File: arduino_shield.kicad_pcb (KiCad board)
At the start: 2 copper layers, 59.1 x 53.3 mm, 33 parts, among them P1 Power, P2 Analog, P3 Digital, P4 Digital, P5 CONN_01X01, P6 CONN_01X01, P7 CONN_01X01, P8 CONN_01X01, U1 MS560702BA03-50

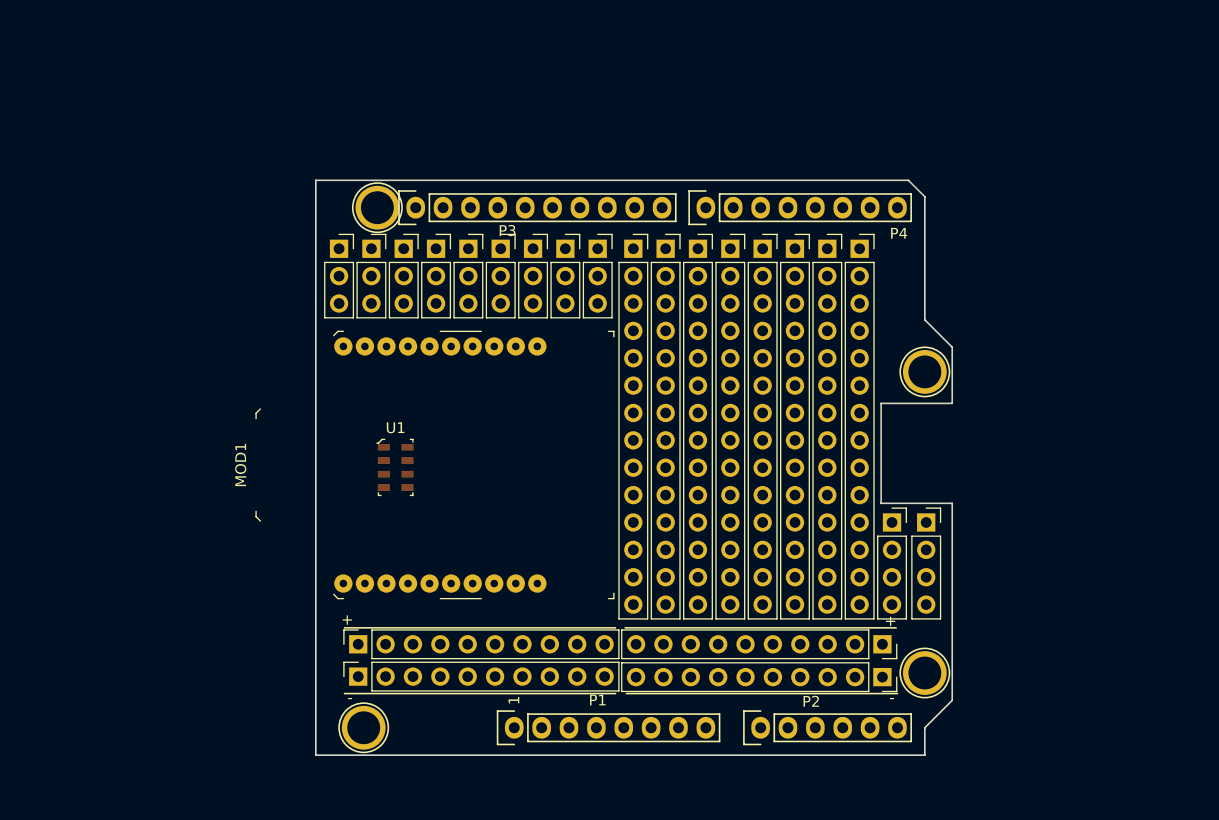
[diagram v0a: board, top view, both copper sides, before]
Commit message: finished maybe?
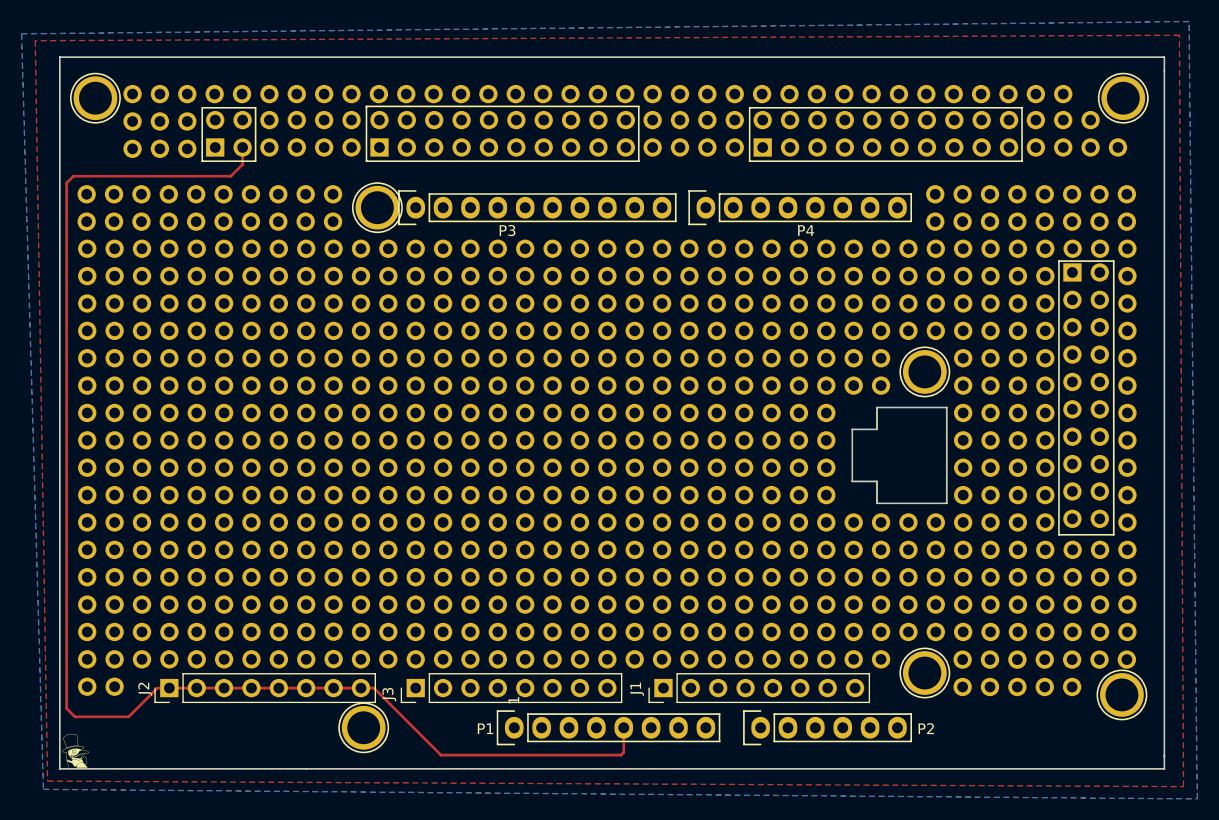
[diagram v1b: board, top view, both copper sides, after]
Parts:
- removed MOD1: XBP9B-DMST-002, digikey-footprints:XBEE_PRO-20_THT
- removed the REF** at (177.2, 104.8)
- removed the REF** at (137.7, 79.4)
- removed the REF** at (134.7, 79.4)
- removed the REF** at (131.7, 79.4)
- removed the REF** at (128.7, 79.4)
- removed the REF** at (125.7, 79.4)
- removed the REF** at (171.0, 79.4)
- removed the REF** at (168.0, 79.4)
- removed the REF** at (165.0, 79.4)
- removed the REF** at (162.0, 79.4)
- removed the REF** at (159.0, 79.4)
- removed the REF** at (174.0, 104.8)
- removed the REF** at (156.0, 79.4)
- removed the REF** at (153.0, 79.4)
- removed the REF** at (150.0, 79.4)
- removed the REF** at (122.7, 79.4)
- removed the REF** at (173.1, 116.1)
- removed the REF** at (173.1, 119.1)
- removed the REF** at (124.5, 119.1)
- removed the REF** at (124.5, 116.1)
- removed the REF** at (146.7, 79.4)
- removed the REF** at (143.7, 79.4)
- removed the REF** at (140.7, 79.4)
- added G***: LOGO, penguin:test106, F.Cu at (98.7, 126.0)
- added J1: GND Rail, Connector_PinHeader_2.54mm:PinHeader_1x08_P2.54mm_Vertical, F.Cu at (152.8, 120.1)
- added J2: 5V Rail, Connector_PinHeader_2.54mm:PinHeader_1x08_P2.54mm_Vertical, F.Cu at (106.9, 120.1)
- added J3: 3v3 Rail, Connector_PinHeader_2.54mm:PinHeader_1x08_P2.54mm_Vertical, F.Cu at (129.8, 120.1)
- added P7: CONN_01X01, Socket_Arduino_Uno:Arduino_1pin, F.Cu at (195.3, 120.8)
- added P7: CONN_01X01, Socket_Arduino_Uno:Arduino_1pin, F.Cu at (195.5, 65.4)
- added P7: CONN_01X01, Socket_Arduino_Uno:Arduino_1pin, F.Cu at (100.1, 65.4)
- added REF**: PROTO_HOLE, One_Month_Footprints:PROTO_HOLE, F.Cu at (101.9, 120.0)
- added REF**: PROTO_HOLE, One_Month_Footprints:PROTO_HOLE, F.Cu at (114.5, 76.9)
- added REF**: PROTO_HOLE, One_Month_Footprints:PROTO_HOLE, F.Cu at (112.0, 97.2)
- added REF**: PROTO_HOLE, One_Month_Footprints:PROTO_HOLE, F.Cu at (109.5, 97.2)
- added REF**: PROTO_HOLE, One_Month_Footprints:PROTO_HOLE, F.Cu at (106.9, 97.2)
- added REF**: PROTO_HOLE, One_Month_Footprints:PROTO_HOLE, F.Cu at (104.4, 97.2)
- added REF**: PROTO_HOLE, One_Month_Footprints:PROTO_HOLE, F.Cu at (101.9, 97.2)
- added REF**: PROTO_HOLE, One_Month_Footprints:PROTO_HOLE, F.Cu at (99.3, 97.2)
- added REF**: PROTO_HOLE, One_Month_Footprints:PROTO_HOLE, F.Cu at (119.6, 94.6)
- added REF**: PROTO_HOLE, One_Month_Footprints:PROTO_HOLE, F.Cu at (117.1, 94.6)
- added REF**: PROTO_HOLE, One_Month_Footprints:PROTO_HOLE, F.Cu at (114.6, 94.6)
- added REF**: PROTO_HOLE, One_Month_Footprints:PROTO_HOLE, F.Cu at (112.0, 94.6)
- added REF**: PROTO_HOLE, One_Month_Footprints:PROTO_HOLE, F.Cu at (109.4, 76.9)
- added REF**: PROTO_HOLE, One_Month_Footprints:PROTO_HOLE, F.Cu at (109.5, 94.6)
- added REF**: PROTO_HOLE, One_Month_Footprints:PROTO_HOLE, F.Cu at (106.9, 94.6)
- added REF**: PROTO_HOLE, One_Month_Footprints:PROTO_HOLE, F.Cu at (104.4, 94.6)
- added REF**: PROTO_HOLE, One_Month_Footprints:PROTO_HOLE, F.Cu at (101.9, 94.6)
- added REF**: PROTO_HOLE, One_Month_Footprints:PROTO_HOLE, F.Cu at (99.3, 94.6)
- added REF**: PROTO_HOLE, One_Month_Footprints:PROTO_HOLE, F.Cu at (119.6, 92.1)
- added REF**: PROTO_HOLE, One_Month_Footprints:PROTO_HOLE, F.Cu at (117.1, 92.1)
- added REF**: PROTO_HOLE, One_Month_Footprints:PROTO_HOLE, F.Cu at (114.6, 92.1)
- added REF**: PROTO_HOLE, One_Month_Footprints:PROTO_HOLE, F.Cu at (112.0, 92.1)
- added REF**: PROTO_HOLE, One_Month_Footprints:PROTO_HOLE, F.Cu at (109.5, 92.1)
- added REF**: PROTO_HOLE, One_Month_Footprints:PROTO_HOLE, F.Cu at (106.9, 76.9)
- added REF**: PROTO_HOLE, One_Month_Footprints:PROTO_HOLE, F.Cu at (106.9, 92.1)
- added REF**: PROTO_HOLE, One_Month_Footprints:PROTO_HOLE, F.Cu at (104.4, 92.1)
- added REF**: PROTO_HOLE, One_Month_Footprints:PROTO_HOLE, F.Cu at (101.9, 92.1)
- added REF**: PROTO_HOLE, One_Month_Footprints:PROTO_HOLE, F.Cu at (99.3, 92.1)
- added REF**: PROTO_HOLE, One_Month_Footprints:PROTO_HOLE, F.Cu at (119.6, 89.5)
- added REF**: PROTO_HOLE, One_Month_Footprints:PROTO_HOLE, F.Cu at (117.1, 89.5)
- added REF**: PROTO_HOLE, One_Month_Footprints:PROTO_HOLE, F.Cu at (114.6, 89.5)
- added REF**: PROTO_HOLE, One_Month_Footprints:PROTO_HOLE, F.Cu at (112.0, 89.5)
- added REF**: PROTO_HOLE, One_Month_Footprints:PROTO_HOLE, F.Cu at (109.5, 89.5)
- added REF**: PROTO_HOLE, One_Month_Footprints:PROTO_HOLE, F.Cu at (106.9, 89.5)
- added REF**: PROTO_HOLE, One_Month_Footprints:PROTO_HOLE, F.Cu at (122.1, 76.9)
- added REF**: PROTO_HOLE, One_Month_Footprints:PROTO_HOLE, F.Cu at (104.4, 89.5)
- added REF**: PROTO_HOLE, One_Month_Footprints:PROTO_HOLE, F.Cu at (101.9, 89.5)
- added REF**: PROTO_HOLE, One_Month_Footprints:PROTO_HOLE, F.Cu at (99.3, 89.5)
- added REF**: PROTO_HOLE, One_Month_Footprints:PROTO_HOLE, F.Cu at (119.6, 87.0)
- added REF**: PROTO_HOLE, One_Month_Footprints:PROTO_HOLE, F.Cu at (117.1, 87.0)
- added REF**: PROTO_HOLE, One_Month_Footprints:PROTO_HOLE, F.Cu at (114.6, 87.0)
- added REF**: PROTO_HOLE, One_Month_Footprints:PROTO_HOLE, F.Cu at (112.0, 87.0)
- added REF**: PROTO_HOLE, One_Month_Footprints:PROTO_HOLE, F.Cu at (109.5, 87.0)
- added REF**: PROTO_HOLE, One_Month_Footprints:PROTO_HOLE, F.Cu at (106.9, 87.0)
- added REF**: PROTO_HOLE, One_Month_Footprints:PROTO_HOLE, F.Cu at (104.4, 87.0)
- added REF**: PROTO_HOLE, One_Month_Footprints:PROTO_HOLE, F.Cu at (119.6, 74.3)
- added REF**: PROTO_HOLE, One_Month_Footprints:PROTO_HOLE, F.Cu at (101.9, 87.0)
- added REF**: PROTO_HOLE, One_Month_Footprints:PROTO_HOLE, F.Cu at (99.3, 87.0)
- added REF**: PROTO_HOLE, One_Month_Footprints:PROTO_HOLE, F.Cu at (119.6, 84.5)
- added REF**: PROTO_HOLE, One_Month_Footprints:PROTO_HOLE, F.Cu at (117.1, 84.5)
- added REF**: PROTO_HOLE, One_Month_Footprints:PROTO_HOLE, F.Cu at (114.6, 84.5)
- added REF**: PROTO_HOLE, One_Month_Footprints:PROTO_HOLE, F.Cu at (112.0, 84.5)
- added REF**: PROTO_HOLE, One_Month_Footprints:PROTO_HOLE, F.Cu at (109.5, 84.5)
- added REF**: PROTO_HOLE, One_Month_Footprints:PROTO_HOLE, F.Cu at (106.9, 84.5)
- added REF**: PROTO_HOLE, One_Month_Footprints:PROTO_HOLE, F.Cu at (104.4, 84.5)
- added REF**: PROTO_HOLE, One_Month_Footprints:PROTO_HOLE, F.Cu at (101.9, 84.5)
- added REF**: PROTO_HOLE, One_Month_Footprints:PROTO_HOLE, F.Cu at (112.0, 74.3)
- added REF**: PROTO_HOLE, One_Month_Footprints:PROTO_HOLE, F.Cu at (99.3, 84.5)
- added REF**: PROTO_HOLE, One_Month_Footprints:PROTO_HOLE, F.Cu at (119.6, 81.9)
- added REF**: PROTO_HOLE, One_Month_Footprints:PROTO_HOLE, F.Cu at (117.1, 81.9)
- added REF**: PROTO_HOLE, One_Month_Footprints:PROTO_HOLE, F.Cu at (114.6, 81.9)
- added REF**: PROTO_HOLE, One_Month_Footprints:PROTO_HOLE, F.Cu at (112.0, 81.9)
- added REF**: PROTO_HOLE, One_Month_Footprints:PROTO_HOLE, F.Cu at (109.5, 81.9)
- added REF**: PROTO_HOLE, One_Month_Footprints:PROTO_HOLE, F.Cu at (106.9, 81.9)
- added REF**: PROTO_HOLE, One_Month_Footprints:PROTO_HOLE, F.Cu at (104.4, 81.9)
- added REF**: PROTO_HOLE, One_Month_Footprints:PROTO_HOLE, F.Cu at (101.9, 81.9)
- added REF**: PROTO_HOLE, One_Month_Footprints:PROTO_HOLE, F.Cu at (99.3, 81.9)
- added REF**: PROTO_HOLE, One_Month_Footprints:PROTO_HOLE, F.Cu at (119.6, 76.9)
- added REF**: PROTO_HOLE, One_Month_Footprints:PROTO_HOLE, F.Cu at (195.8, 79.4)
- added REF**: PROTO_HOLE, One_Month_Footprints:PROTO_HOLE, F.Cu at (193.3, 79.4)
- added REF**: PROTO_HOLE, One_Month_Footprints:PROTO_HOLE, F.Cu at (190.8, 79.4)
- added REF**: PROTO_HOLE, One_Month_Footprints:PROTO_HOLE, F.Cu at (188.2, 79.4)
- added REF**: PROTO_HOLE, One_Month_Footprints:PROTO_HOLE, F.Cu at (185.7, 79.4)
- added REF**: PROTO_HOLE, One_Month_Footprints:PROTO_HOLE, F.Cu at (183.1, 79.4)
- added REF**: PROTO_HOLE, One_Month_Footprints:PROTO_HOLE, F.Cu at (180.6, 79.4)
- added REF**: PROTO_HOLE, One_Month_Footprints:PROTO_HOLE, F.Cu at (178.1, 79.4)
- added REF**: PROTO_HOLE, One_Month_Footprints:PROTO_HOLE, F.Cu at (175.5, 79.4)
- added REF**: PROTO_HOLE, One_Month_Footprints:PROTO_HOLE, F.Cu at (173.0, 79.4)
- added REF**: PROTO_HOLE, One_Month_Footprints:PROTO_HOLE, F.Cu at (109.4, 74.3)
- added REF**: PROTO_HOLE, One_Month_Footprints:PROTO_HOLE, F.Cu at (170.4, 79.4)
- added REF**: PROTO_HOLE, One_Month_Footprints:PROTO_HOLE, F.Cu at (167.9, 79.4)
- added REF**: PROTO_HOLE, One_Month_Footprints:PROTO_HOLE, F.Cu at (165.4, 79.4)
- added REF**: PROTO_HOLE, One_Month_Footprints:PROTO_HOLE, F.Cu at (162.8, 79.4)
- added REF**: PROTO_HOLE, One_Month_Footprints:PROTO_HOLE, F.Cu at (160.3, 79.4)
- added REF**: PROTO_HOLE, One_Month_Footprints:PROTO_HOLE, F.Cu at (157.7, 79.4)
- added REF**: PROTO_HOLE, One_Month_Footprints:PROTO_HOLE, F.Cu at (155.2, 79.4)
- added REF**: PROTO_HOLE, One_Month_Footprints:PROTO_HOLE, F.Cu at (152.7, 79.4)
- added REF**: PROTO_HOLE, One_Month_Footprints:PROTO_HOLE, F.Cu at (150.1, 79.4)
- added REF**: PROTO_HOLE, One_Month_Footprints:PROTO_HOLE, F.Cu at (147.6, 79.4)
- added REF**: PROTO_HOLE, One_Month_Footprints:PROTO_HOLE, F.Cu at (117.0, 76.9)
- added REF**: PROTO_HOLE, One_Month_Footprints:PROTO_HOLE, F.Cu at (145.0, 79.4)
- added REF**: PROTO_HOLE, One_Month_Footprints:PROTO_HOLE, F.Cu at (142.5, 79.4)
- added REF**: PROTO_HOLE, One_Month_Footprints:PROTO_HOLE, F.Cu at (140.0, 79.4)
- added REF**: PROTO_HOLE, One_Month_Footprints:PROTO_HOLE, F.Cu at (137.4, 79.4)
- added REF**: PROTO_HOLE, One_Month_Footprints:PROTO_HOLE, F.Cu at (134.9, 79.4)
- added REF**: PROTO_HOLE, One_Month_Footprints:PROTO_HOLE, F.Cu at (132.3, 79.4)
- added REF**: PROTO_HOLE, One_Month_Footprints:PROTO_HOLE, F.Cu at (129.8, 79.4)
- added REF**: PROTO_HOLE, One_Month_Footprints:PROTO_HOLE, F.Cu at (127.3, 79.4)
- added REF**: PROTO_HOLE, One_Month_Footprints:PROTO_HOLE, F.Cu at (124.7, 79.4)
- added REF**: PROTO_HOLE, One_Month_Footprints:PROTO_HOLE, F.Cu at (122.2, 79.4)
- added REF**: PROTO_HOLE, One_Month_Footprints:PROTO_HOLE, F.Cu at (117.0, 74.3)
- added REF**: PROTO_HOLE, One_Month_Footprints:PROTO_HOLE, F.Cu at (119.6, 79.4)
- added REF**: PROTO_HOLE, One_Month_Footprints:PROTO_HOLE, F.Cu at (117.1, 79.4)
- added REF**: PROTO_HOLE, One_Month_Footprints:PROTO_HOLE, F.Cu at (114.6, 79.4)
- added REF**: PROTO_HOLE, One_Month_Footprints:PROTO_HOLE, F.Cu at (112.0, 79.4)
- added REF**: PROTO_HOLE, One_Month_Footprints:PROTO_HOLE, F.Cu at (109.5, 79.4)
- added REF**: PROTO_HOLE, One_Month_Footprints:PROTO_HOLE, F.Cu at (106.9, 79.4)
- added REF**: PROTO_HOLE, One_Month_Footprints:PROTO_HOLE, F.Cu at (104.4, 79.4)
- added REF**: PROTO_HOLE, One_Month_Footprints:PROTO_HOLE, F.Cu at (101.9, 79.4)
- added REF**: PROTO_HOLE, One_Month_Footprints:PROTO_HOLE, F.Cu at (99.3, 79.4)
- added REF**: PROTO_HOLE, One_Month_Footprints:PROTO_HOLE, F.Cu at (190.7, 120.0)
- added REF**: PROTO_HOLE, One_Month_Footprints:PROTO_HOLE, F.Cu at (99.3, 120.0)
- added REF**: PROTO_HOLE, One_Month_Footprints:PROTO_HOLE, F.Cu at (122.1, 74.3)
- added REF**: PROTO_HOLE, One_Month_Footprints:PROTO_HOLE, F.Cu at (188.2, 120.0)
- added REF**: PROTO_HOLE, One_Month_Footprints:PROTO_HOLE, F.Cu at (185.6, 120.0)
- added REF**: PROTO_HOLE, One_Month_Footprints:PROTO_HOLE, F.Cu at (183.1, 120.0)
- added REF**: PROTO_HOLE, One_Month_Footprints:PROTO_HOLE, F.Cu at (180.5, 120.0)
- added REF**: PROTO_HOLE, One_Month_Footprints:PROTO_HOLE, F.Cu at (195.8, 74.3)
- added REF**: PROTO_HOLE, One_Month_Footprints:PROTO_HOLE, F.Cu at (193.2, 74.3)
- added REF**: PROTO_HOLE, One_Month_Footprints:PROTO_HOLE, F.Cu at (190.7, 74.3)
- added REF**: PROTO_HOLE, One_Month_Footprints:PROTO_HOLE, F.Cu at (188.2, 74.3)
- added REF**: PROTO_HOLE, One_Month_Footprints:PROTO_HOLE, F.Cu at (185.6, 74.3)
- added REF**: PROTO_HOLE, One_Month_Footprints:PROTO_HOLE, F.Cu at (183.1, 74.3)
- added REF**: PROTO_HOLE, One_Month_Footprints:PROTO_HOLE, F.Cu at (114.5, 74.3)
- added REF**: PROTO_HOLE, One_Month_Footprints:PROTO_HOLE, F.Cu at (180.5, 74.3)
- added REF**: PROTO_HOLE, One_Month_Footprints:PROTO_HOLE, F.Cu at (195.8, 76.9)
- added REF**: PROTO_HOLE, One_Month_Footprints:PROTO_HOLE, F.Cu at (193.2, 76.9)
- added REF**: PROTO_HOLE, One_Month_Footprints:PROTO_HOLE, F.Cu at (190.7, 76.9)
- added REF**: PROTO_HOLE, One_Month_Footprints:PROTO_HOLE, F.Cu at (188.2, 76.9)
- added REF**: PROTO_HOLE, One_Month_Footprints:PROTO_HOLE, F.Cu at (185.6, 76.9)
- added REF**: PROTO_HOLE, One_Month_Footprints:PROTO_HOLE, F.Cu at (183.1, 76.9)
- added REF**: PROTO_HOLE, One_Month_Footprints:PROTO_HOLE, F.Cu at (180.5, 76.9)
- added REF**: PROTO_HOLE, One_Month_Footprints:PROTO_HOLE, F.Cu at (178.0, 74.3)
- added REF**: PROTO_HOLE, One_Month_Footprints:PROTO_HOLE, F.Cu at (178.0, 76.9)
- added REF**: PROTO_HOLE, One_Month_Footprints:PROTO_HOLE, F.Cu at (104.3, 74.3)
- added REF**: PROTO_HOLE, One_Month_Footprints:PROTO_HOLE, F.Cu at (195.8, 117.5)
- added REF**: PROTO_HOLE, One_Month_Footprints:PROTO_HOLE, F.Cu at (193.2, 117.5)
- added REF**: PROTO_HOLE, One_Month_Footprints:PROTO_HOLE, F.Cu at (190.7, 117.5)
- added REF**: PROTO_HOLE, One_Month_Footprints:PROTO_HOLE, F.Cu at (188.2, 117.5)
- added REF**: PROTO_HOLE, One_Month_Footprints:PROTO_HOLE, F.Cu at (185.6, 117.5)
- added REF**: PROTO_HOLE, One_Month_Footprints:PROTO_HOLE, F.Cu at (183.1, 117.5)
- added REF**: PROTO_HOLE, One_Month_Footprints:PROTO_HOLE, F.Cu at (180.5, 117.5)
- added REF**: PROTO_HOLE, One_Month_Footprints:PROTO_HOLE, F.Cu at (195.0, 70.0)
- added REF**: PROTO_HOLE, One_Month_Footprints:PROTO_HOLE, F.Cu at (192.4, 70.0)
- added REF**: PROTO_HOLE, One_Month_Footprints:PROTO_HOLE, F.Cu at (189.9, 70.0)
- added REF**: PROTO_HOLE, One_Month_Footprints:PROTO_HOLE, F.Cu at (122.2, 117.4)
- added REF**: PROTO_HOLE, One_Month_Footprints:PROTO_HOLE, F.Cu at (187.3, 70.0)
- added REF**: PROTO_HOLE, One_Month_Footprints:PROTO_HOLE, F.Cu at (192.4, 67.4)
- added REF**: PROTO_HOLE, One_Month_Footprints:PROTO_HOLE, F.Cu at (189.9, 67.4)
- added REF**: PROTO_HOLE, One_Month_Footprints:PROTO_HOLE, F.Cu at (187.3, 67.4)
- added REF**: PROTO_HOLE, One_Month_Footprints:PROTO_HOLE, F.Cu at (159.4, 70.0)
- added REF**: PROTO_HOLE, One_Month_Footprints:PROTO_HOLE, F.Cu at (156.9, 70.0)
- added REF**: PROTO_HOLE, One_Month_Footprints:PROTO_HOLE, F.Cu at (154.3, 70.0)
- added REF**: PROTO_HOLE, One_Month_Footprints:PROTO_HOLE, F.Cu at (151.8, 70.0)
- added REF**: PROTO_HOLE, One_Month_Footprints:PROTO_HOLE, F.Cu at (159.4, 67.4)
- added REF**: PROTO_HOLE, One_Month_Footprints:PROTO_HOLE, F.Cu at (156.9, 67.4)
- added REF**: PROTO_HOLE, One_Month_Footprints:PROTO_HOLE, F.Cu at (122.2, 114.9)
- added REF**: PROTO_HOLE, One_Month_Footprints:PROTO_HOLE, F.Cu at (154.3, 67.4)
- added REF**: PROTO_HOLE, One_Month_Footprints:PROTO_HOLE, F.Cu at (151.8, 67.4)
- added REF**: PROTO_HOLE, One_Month_Footprints:PROTO_HOLE, F.Cu at (123.8, 70.0)
- added REF**: PROTO_HOLE, One_Month_Footprints:PROTO_HOLE, F.Cu at (121.3, 70.0)
- added REF**: PROTO_HOLE, One_Month_Footprints:PROTO_HOLE, F.Cu at (118.8, 70.0)
- added REF**: PROTO_HOLE, One_Month_Footprints:PROTO_HOLE, F.Cu at (116.2, 70.0)
- added REF**: PROTO_HOLE, One_Month_Footprints:PROTO_HOLE, F.Cu at (123.8, 67.4)
- added REF**: PROTO_HOLE, One_Month_Footprints:PROTO_HOLE, F.Cu at (121.3, 67.4)
- added REF**: PROTO_HOLE, One_Month_Footprints:PROTO_HOLE, F.Cu at (118.8, 67.4)
- added REF**: PROTO_HOLE, One_Month_Footprints:PROTO_HOLE, F.Cu at (116.2, 67.4)
- added REF**: PROTO_HOLE, One_Month_Footprints:PROTO_HOLE, F.Cu at (119.6, 117.5)
- added REF**: PROTO_HOLE, One_Month_Footprints:PROTO_HOLE, F.Cu at (189.9, 65.0)
- added REF**: PROTO_HOLE, One_Month_Footprints:PROTO_HOLE, F.Cu at (187.3, 65.0)
- added REF**: PROTO_HOLE, One_Month_Footprints:PROTO_HOLE, F.Cu at (184.8, 65.0)
- added REF**: PROTO_HOLE, One_Month_Footprints:PROTO_HOLE, F.Cu at (182.3, 65.0)
- added REF**: PROTO_HOLE, One_Month_Footprints:PROTO_HOLE, F.Cu at (179.7, 65.0)
- added REF**: PROTO_HOLE, One_Month_Footprints:PROTO_HOLE, F.Cu at (177.2, 65.0)
- added REF**: PROTO_HOLE, One_Month_Footprints:PROTO_HOLE, F.Cu at (174.6, 65.0)
- added REF**: PROTO_HOLE, One_Month_Footprints:PROTO_HOLE, F.Cu at (172.1, 65.0)
- added REF**: PROTO_HOLE, One_Month_Footprints:PROTO_HOLE, F.Cu at (169.6, 65.0)
- added REF**: PROTO_HOLE, One_Month_Footprints:PROTO_HOLE, F.Cu at (167.0, 65.0)
- added REF**: PROTO_HOLE, One_Month_Footprints:PROTO_HOLE, F.Cu at (117.1, 117.5)
- added REF**: PROTO_HOLE, One_Month_Footprints:PROTO_HOLE, F.Cu at (164.5, 65.0)
- added REF**: PROTO_HOLE, One_Month_Footprints:PROTO_HOLE, F.Cu at (161.9, 65.0)
- added REF**: PROTO_HOLE, One_Month_Footprints:PROTO_HOLE, F.Cu at (159.4, 65.0)
- added REF**: PROTO_HOLE, One_Month_Footprints:PROTO_HOLE, F.Cu at (156.9, 65.0)
- added REF**: PROTO_HOLE, One_Month_Footprints:PROTO_HOLE, F.Cu at (154.3, 65.0)
- added REF**: PROTO_HOLE, One_Month_Footprints:PROTO_HOLE, F.Cu at (151.8, 65.0)
- added REF**: PROTO_HOLE, One_Month_Footprints:PROTO_HOLE, F.Cu at (149.2, 65.0)
- added REF**: PROTO_HOLE, One_Month_Footprints:PROTO_HOLE, F.Cu at (146.7, 65.0)
- added REF**: PROTO_HOLE, One_Month_Footprints:PROTO_HOLE, F.Cu at (144.2, 65.0)
- added REF**: PROTO_HOLE, One_Month_Footprints:PROTO_HOLE, F.Cu at (141.6, 65.0)
- added REF**: PROTO_HOLE, One_Month_Footprints:PROTO_HOLE, F.Cu at (114.6, 117.5)
- added REF**: PROTO_HOLE, One_Month_Footprints:PROTO_HOLE, F.Cu at (139.1, 65.0)
- added REF**: PROTO_HOLE, One_Month_Footprints:PROTO_HOLE, F.Cu at (136.5, 65.0)
- added REF**: PROTO_HOLE, One_Month_Footprints:PROTO_HOLE, F.Cu at (134.0, 65.0)
- added REF**: PROTO_HOLE, One_Month_Footprints:PROTO_HOLE, F.Cu at (131.5, 65.0)
- added REF**: PROTO_HOLE, One_Month_Footprints:PROTO_HOLE, F.Cu at (128.9, 65.0)
- added REF**: PROTO_HOLE, One_Month_Footprints:PROTO_HOLE, F.Cu at (126.4, 65.0)
- added REF**: PROTO_HOLE, One_Month_Footprints:PROTO_HOLE, F.Cu at (123.8, 65.0)
- added REF**: PROTO_HOLE, One_Month_Footprints:PROTO_HOLE, F.Cu at (121.3, 65.0)
- added REF**: PROTO_HOLE, One_Month_Footprints:PROTO_HOLE, F.Cu at (118.8, 65.0)
- added REF**: PROTO_HOLE, One_Month_Footprints:PROTO_HOLE, F.Cu at (116.2, 65.0)
- added REF**: PROTO_HOLE, One_Month_Footprints:PROTO_HOLE, F.Cu at (112.0, 117.5)
- added REF**: PROTO_HOLE, One_Month_Footprints:PROTO_HOLE, F.Cu at (113.7, 65.0)
- added REF**: PROTO_HOLE, One_Month_Footprints:PROTO_HOLE, F.Cu at (111.1, 65.0)
- added REF**: PROTO_HOLE, One_Month_Footprints:PROTO_HOLE, F.Cu at (108.6, 65.0)
- added REF**: PROTO_HOLE, One_Month_Footprints:PROTO_HOLE, F.Cu at (106.1, 65.0)
- added REF**: PROTO_HOLE, One_Month_Footprints:PROTO_HOLE, F.Cu at (103.5, 65.0)
- added REF**: PROTO_HOLE, One_Month_Footprints:PROTO_HOLE, F.Cu at (108.6, 70.1)
- added REF**: PROTO_HOLE, One_Month_Footprints:PROTO_HOLE, F.Cu at (106.1, 70.1)
- added REF**: PROTO_HOLE, One_Month_Footprints:PROTO_HOLE, F.Cu at (103.5, 70.1)
- added REF**: PROTO_HOLE, One_Month_Footprints:PROTO_HOLE, F.Cu at (108.6, 67.6)
- added REF**: PROTO_HOLE, One_Month_Footprints:PROTO_HOLE, F.Cu at (106.1, 67.6)
- added REF**: PROTO_HOLE, One_Month_Footprints:PROTO_HOLE, F.Cu at (109.5, 117.5)
- added REF**: PROTO_HOLE, One_Month_Footprints:PROTO_HOLE, F.Cu at (103.5, 67.6)
- added REF**: PROTO_HOLE, One_Month_Footprints:PROTO_HOLE, F.Cu at (195.8, 104.8)
- added REF**: PROTO_HOLE, One_Month_Footprints:PROTO_HOLE, F.Cu at (195.8, 102.2)
- added REF**: PROTO_HOLE, One_Month_Footprints:PROTO_HOLE, F.Cu at (195.8, 99.7)
- added REF**: PROTO_HOLE, One_Month_Footprints:PROTO_HOLE, F.Cu at (195.8, 97.2)
- added REF**: PROTO_HOLE, One_Month_Footprints:PROTO_HOLE, F.Cu at (195.8, 94.6)
- added REF**: PROTO_HOLE, One_Month_Footprints:PROTO_HOLE, F.Cu at (195.8, 92.1)
- added REF**: PROTO_HOLE, One_Month_Footprints:PROTO_HOLE, F.Cu at (195.8, 89.5)
- added REF**: PROTO_HOLE, One_Month_Footprints:PROTO_HOLE, F.Cu at (195.8, 87.0)
- added REF**: PROTO_HOLE, One_Month_Footprints:PROTO_HOLE, F.Cu at (195.8, 84.5)
- added REF**: PROTO_HOLE, One_Month_Footprints:PROTO_HOLE, F.Cu at (101.8, 76.9)
- added REF**: PROTO_HOLE, One_Month_Footprints:PROTO_HOLE, F.Cu at (106.9, 117.5)
- added REF**: PROTO_HOLE, One_Month_Footprints:PROTO_HOLE, F.Cu at (195.8, 81.9)
- added REF**: PROTO_HOLE, One_Month_Footprints:PROTO_HOLE, F.Cu at (188.2, 102.2)
- added REF**: PROTO_HOLE, One_Month_Footprints:PROTO_HOLE, F.Cu at (185.7, 102.2)
- added REF**: PROTO_HOLE, One_Month_Footprints:PROTO_HOLE, F.Cu at (183.1, 102.2)
- added REF**: PROTO_HOLE, One_Month_Footprints:PROTO_HOLE, F.Cu at (180.6, 102.2)
- added REF**: PROTO_HOLE, One_Month_Footprints:PROTO_HOLE, F.Cu at (188.2, 99.7)
- added REF**: PROTO_HOLE, One_Month_Footprints:PROTO_HOLE, F.Cu at (185.7, 99.7)
- added REF**: PROTO_HOLE, One_Month_Footprints:PROTO_HOLE, F.Cu at (183.1, 99.7)
- added REF**: PROTO_HOLE, One_Month_Footprints:PROTO_HOLE, F.Cu at (180.6, 99.7)
- added REF**: PROTO_HOLE, One_Month_Footprints:PROTO_HOLE, F.Cu at (188.2, 97.2)
- added REF**: PROTO_HOLE, One_Month_Footprints:PROTO_HOLE, F.Cu at (104.4, 117.5)
- added REF**: PROTO_HOLE, One_Month_Footprints:PROTO_HOLE, F.Cu at (185.7, 97.2)
- added REF**: PROTO_HOLE, One_Month_Footprints:PROTO_HOLE, F.Cu at (183.1, 97.2)
- added REF**: PROTO_HOLE, One_Month_Footprints:PROTO_HOLE, F.Cu at (180.6, 97.2)
- added REF**: PROTO_HOLE, One_Month_Footprints:PROTO_HOLE, F.Cu at (188.2, 94.6)
- added REF**: PROTO_HOLE, One_Month_Footprints:PROTO_HOLE, F.Cu at (185.7, 94.6)
- added REF**: PROTO_HOLE, One_Month_Footprints:PROTO_HOLE, F.Cu at (183.1, 94.6)
- added REF**: PROTO_HOLE, One_Month_Footprints:PROTO_HOLE, F.Cu at (180.6, 94.6)
- added REF**: PROTO_HOLE, One_Month_Footprints:PROTO_HOLE, F.Cu at (188.2, 92.1)
- added REF**: PROTO_HOLE, One_Month_Footprints:PROTO_HOLE, F.Cu at (185.7, 92.1)
- added REF**: PROTO_HOLE, One_Month_Footprints:PROTO_HOLE, F.Cu at (183.1, 92.1)
- added REF**: PROTO_HOLE, One_Month_Footprints:PROTO_HOLE, F.Cu at (101.9, 117.5)
- added REF**: PROTO_HOLE, One_Month_Footprints:PROTO_HOLE, F.Cu at (180.6, 92.1)
- added REF**: PROTO_HOLE, One_Month_Footprints:PROTO_HOLE, F.Cu at (188.2, 89.5)
- added REF**: PROTO_HOLE, One_Month_Footprints:PROTO_HOLE, F.Cu at (185.7, 89.5)
- added REF**: PROTO_HOLE, One_Month_Footprints:PROTO_HOLE, F.Cu at (183.1, 89.5)
- added REF**: PROTO_HOLE, One_Month_Footprints:PROTO_HOLE, F.Cu at (180.6, 89.5)
- added REF**: PROTO_HOLE, One_Month_Footprints:PROTO_HOLE, F.Cu at (173.0, 117.5)
- added REF**: PROTO_HOLE, One_Month_Footprints:PROTO_HOLE, F.Cu at (170.4, 117.5)
- added REF**: PROTO_HOLE, One_Month_Footprints:PROTO_HOLE, F.Cu at (167.9, 117.5)
- added REF**: PROTO_HOLE, One_Month_Footprints:PROTO_HOLE, F.Cu at (165.4, 117.5)
- added REF**: PROTO_HOLE, One_Month_Footprints:PROTO_HOLE, F.Cu at (162.8, 117.5)
- added REF**: PROTO_HOLE, One_Month_Footprints:PROTO_HOLE, F.Cu at (99.3, 117.5)
- added REF**: PROTO_HOLE, One_Month_Footprints:PROTO_HOLE, F.Cu at (160.3, 117.5)
- added REF**: PROTO_HOLE, One_Month_Footprints:PROTO_HOLE, F.Cu at (157.7, 117.5)
- added REF**: PROTO_HOLE, One_Month_Footprints:PROTO_HOLE, F.Cu at (155.2, 117.5)
- added REF**: PROTO_HOLE, One_Month_Footprints:PROTO_HOLE, F.Cu at (152.7, 117.5)
- added REF**: PROTO_HOLE, One_Month_Footprints:PROTO_HOLE, F.Cu at (150.1, 117.5)
- added REF**: PROTO_HOLE, One_Month_Footprints:PROTO_HOLE, F.Cu at (147.6, 117.5)
- added REF**: PROTO_HOLE, One_Month_Footprints:PROTO_HOLE, F.Cu at (145.0, 117.5)
- added REF**: PROTO_HOLE, One_Month_Footprints:PROTO_HOLE, F.Cu at (142.5, 117.5)
- added REF**: PROTO_HOLE, One_Month_Footprints:PROTO_HOLE, F.Cu at (140.0, 117.5)
- added REF**: PROTO_HOLE, One_Month_Footprints:PROTO_HOLE, F.Cu at (137.4, 117.5)
- added REF**: PROTO_HOLE, One_Month_Footprints:PROTO_HOLE, F.Cu at (119.6, 114.9)
- added REF**: PROTO_HOLE, One_Month_Footprints:PROTO_HOLE, F.Cu at (134.9, 117.5)
- added REF**: PROTO_HOLE, One_Month_Footprints:PROTO_HOLE, F.Cu at (132.3, 117.5)
- added REF**: PROTO_HOLE, One_Month_Footprints:PROTO_HOLE, F.Cu at (129.8, 117.5)
- added REF**: PROTO_HOLE, One_Month_Footprints:PROTO_HOLE, F.Cu at (127.3, 117.5)
- added REF**: PROTO_HOLE, One_Month_Footprints:PROTO_HOLE, F.Cu at (124.7, 117.5)
- added REF**: PROTO_HOLE, One_Month_Footprints:PROTO_HOLE, F.Cu at (195.8, 114.9)
- added REF**: PROTO_HOLE, One_Month_Footprints:PROTO_HOLE, F.Cu at (193.3, 114.9)
- added REF**: PROTO_HOLE, One_Month_Footprints:PROTO_HOLE, F.Cu at (190.8, 114.9)
- added REF**: PROTO_HOLE, One_Month_Footprints:PROTO_HOLE, F.Cu at (188.2, 114.9)
- added REF**: PROTO_HOLE, One_Month_Footprints:PROTO_HOLE, F.Cu at (185.7, 114.9)
- added REF**: PROTO_HOLE, One_Month_Footprints:PROTO_HOLE, F.Cu at (117.1, 114.9)
- added REF**: PROTO_HOLE, One_Month_Footprints:PROTO_HOLE, F.Cu at (183.1, 114.9)
- added REF**: PROTO_HOLE, One_Month_Footprints:PROTO_HOLE, F.Cu at (180.6, 114.9)
- added REF**: PROTO_HOLE, One_Month_Footprints:PROTO_HOLE, F.Cu at (178.1, 114.9)
- added REF**: PROTO_HOLE, One_Month_Footprints:PROTO_HOLE, F.Cu at (175.5, 114.9)
- added REF**: PROTO_HOLE, One_Month_Footprints:PROTO_HOLE, F.Cu at (173.0, 114.9)
- added REF**: PROTO_HOLE, One_Month_Footprints:PROTO_HOLE, F.Cu at (170.4, 114.9)
- added REF**: PROTO_HOLE, One_Month_Footprints:PROTO_HOLE, F.Cu at (167.9, 114.9)
- added REF**: PROTO_HOLE, One_Month_Footprints:PROTO_HOLE, F.Cu at (165.4, 114.9)
- added REF**: PROTO_HOLE, One_Month_Footprints:PROTO_HOLE, F.Cu at (162.8, 114.9)
- added REF**: PROTO_HOLE, One_Month_Footprints:PROTO_HOLE, F.Cu at (160.3, 114.9)
- added REF**: PROTO_HOLE, One_Month_Footprints:PROTO_HOLE, F.Cu at (114.6, 114.9)
- added REF**: PROTO_HOLE, One_Month_Footprints:PROTO_HOLE, F.Cu at (157.7, 114.9)
- added REF**: PROTO_HOLE, One_Month_Footprints:PROTO_HOLE, F.Cu at (155.2, 114.9)
- added REF**: PROTO_HOLE, One_Month_Footprints:PROTO_HOLE, F.Cu at (152.7, 114.9)
- added REF**: PROTO_HOLE, One_Month_Footprints:PROTO_HOLE, F.Cu at (150.1, 114.9)
- added REF**: PROTO_HOLE, One_Month_Footprints:PROTO_HOLE, F.Cu at (147.6, 114.9)
- added REF**: PROTO_HOLE, One_Month_Footprints:PROTO_HOLE, F.Cu at (145.0, 114.9)
- added REF**: PROTO_HOLE, One_Month_Footprints:PROTO_HOLE, F.Cu at (142.5, 114.9)
- added REF**: PROTO_HOLE, One_Month_Footprints:PROTO_HOLE, F.Cu at (140.0, 114.9)
- added REF**: PROTO_HOLE, One_Month_Footprints:PROTO_HOLE, F.Cu at (137.4, 114.9)
- added REF**: PROTO_HOLE, One_Month_Footprints:PROTO_HOLE, F.Cu at (134.9, 114.9)
- added REF**: PROTO_HOLE, One_Month_Footprints:PROTO_HOLE, F.Cu at (112.0, 114.9)
- added REF**: PROTO_HOLE, One_Month_Footprints:PROTO_HOLE, F.Cu at (132.3, 114.9)
- added REF**: PROTO_HOLE, One_Month_Footprints:PROTO_HOLE, F.Cu at (129.8, 114.9)
- added REF**: PROTO_HOLE, One_Month_Footprints:PROTO_HOLE, F.Cu at (127.3, 114.9)
- added REF**: PROTO_HOLE, One_Month_Footprints:PROTO_HOLE, F.Cu at (124.7, 114.9)
- added REF**: PROTO_HOLE, One_Month_Footprints:PROTO_HOLE, F.Cu at (195.8, 112.4)
- added REF**: PROTO_HOLE, One_Month_Footprints:PROTO_HOLE, F.Cu at (193.3, 112.4)
- added REF**: PROTO_HOLE, One_Month_Footprints:PROTO_HOLE, F.Cu at (190.8, 112.4)
- added REF**: PROTO_HOLE, One_Month_Footprints:PROTO_HOLE, F.Cu at (188.2, 112.4)
- added REF**: PROTO_HOLE, One_Month_Footprints:PROTO_HOLE, F.Cu at (185.7, 112.4)
- added REF**: PROTO_HOLE, One_Month_Footprints:PROTO_HOLE, F.Cu at (183.1, 112.4)
- added REF**: PROTO_HOLE, One_Month_Footprints:PROTO_HOLE, F.Cu at (109.5, 114.9)
- added REF**: PROTO_HOLE, One_Month_Footprints:PROTO_HOLE, F.Cu at (180.6, 112.4)
- added REF**: PROTO_HOLE, One_Month_Footprints:PROTO_HOLE, F.Cu at (178.1, 112.4)
- added REF**: PROTO_HOLE, One_Month_Footprints:PROTO_HOLE, F.Cu at (175.5, 112.4)
- added REF**: PROTO_HOLE, One_Month_Footprints:PROTO_HOLE, F.Cu at (173.0, 112.4)
- added REF**: PROTO_HOLE, One_Month_Footprints:PROTO_HOLE, F.Cu at (170.4, 112.4)
- added REF**: PROTO_HOLE, One_Month_Footprints:PROTO_HOLE, F.Cu at (167.9, 112.4)
- added REF**: PROTO_HOLE, One_Month_Footprints:PROTO_HOLE, F.Cu at (165.4, 112.4)
- added REF**: PROTO_HOLE, One_Month_Footprints:PROTO_HOLE, F.Cu at (162.8, 112.4)
- added REF**: PROTO_HOLE, One_Month_Footprints:PROTO_HOLE, F.Cu at (160.3, 112.4)
- added REF**: PROTO_HOLE, One_Month_Footprints:PROTO_HOLE, F.Cu at (157.7, 112.4)
- added REF**: PROTO_HOLE, One_Month_Footprints:PROTO_HOLE, F.Cu at (106.9, 114.9)
- added REF**: PROTO_HOLE, One_Month_Footprints:PROTO_HOLE, F.Cu at (155.2, 112.4)
- added REF**: PROTO_HOLE, One_Month_Footprints:PROTO_HOLE, F.Cu at (152.7, 112.4)
- added REF**: PROTO_HOLE, One_Month_Footprints:PROTO_HOLE, F.Cu at (150.1, 112.4)
- added REF**: PROTO_HOLE, One_Month_Footprints:PROTO_HOLE, F.Cu at (147.6, 112.4)
- added REF**: PROTO_HOLE, One_Month_Footprints:PROTO_HOLE, F.Cu at (145.0, 112.4)
- added REF**: PROTO_HOLE, One_Month_Footprints:PROTO_HOLE, F.Cu at (142.5, 112.4)
- added REF**: PROTO_HOLE, One_Month_Footprints:PROTO_HOLE, F.Cu at (140.0, 112.4)
- added REF**: PROTO_HOLE, One_Month_Footprints:PROTO_HOLE, F.Cu at (137.4, 112.4)
- added REF**: PROTO_HOLE, One_Month_Footprints:PROTO_HOLE, F.Cu at (134.9, 112.4)
- added REF**: PROTO_HOLE, One_Month_Footprints:PROTO_HOLE, F.Cu at (132.3, 112.4)
- added REF**: PROTO_HOLE, One_Month_Footprints:PROTO_HOLE, F.Cu at (99.3, 74.3)
- added REF**: PROTO_HOLE, One_Month_Footprints:PROTO_HOLE, F.Cu at (104.4, 114.9)
- added REF**: PROTO_HOLE, One_Month_Footprints:PROTO_HOLE, F.Cu at (129.8, 112.4)
- added REF**: PROTO_HOLE, One_Month_Footprints:PROTO_HOLE, F.Cu at (127.3, 112.4)
- added REF**: PROTO_HOLE, One_Month_Footprints:PROTO_HOLE, F.Cu at (124.7, 112.4)
- added REF**: PROTO_HOLE, One_Month_Footprints:PROTO_HOLE, F.Cu at (122.2, 112.4)
- added REF**: PROTO_HOLE, One_Month_Footprints:PROTO_HOLE, F.Cu at (195.8, 109.9)
- added REF**: PROTO_HOLE, One_Month_Footprints:PROTO_HOLE, F.Cu at (193.3, 109.9)
- added REF**: PROTO_HOLE, One_Month_Footprints:PROTO_HOLE, F.Cu at (190.8, 109.9)
- added REF**: PROTO_HOLE, One_Month_Footprints:PROTO_HOLE, F.Cu at (188.2, 109.9)
- added REF**: PROTO_HOLE, One_Month_Footprints:PROTO_HOLE, F.Cu at (185.7, 109.9)
- added REF**: PROTO_HOLE, One_Month_Footprints:PROTO_HOLE, F.Cu at (183.1, 109.9)
- added REF**: PROTO_HOLE, One_Month_Footprints:PROTO_HOLE, F.Cu at (101.9, 114.9)
- added REF**: PROTO_HOLE, One_Month_Footprints:PROTO_HOLE, F.Cu at (180.6, 109.9)
- added REF**: PROTO_HOLE, One_Month_Footprints:PROTO_HOLE, F.Cu at (178.1, 109.9)
- added REF**: PROTO_HOLE, One_Month_Footprints:PROTO_HOLE, F.Cu at (175.5, 109.9)
- added REF**: PROTO_HOLE, One_Month_Footprints:PROTO_HOLE, F.Cu at (173.0, 109.9)
- added REF**: PROTO_HOLE, One_Month_Footprints:PROTO_HOLE, F.Cu at (170.4, 109.9)
- added REF**: PROTO_HOLE, One_Month_Footprints:PROTO_HOLE, F.Cu at (167.9, 109.9)
- added REF**: PROTO_HOLE, One_Month_Footprints:PROTO_HOLE, F.Cu at (165.4, 109.9)
- added REF**: PROTO_HOLE, One_Month_Footprints:PROTO_HOLE, F.Cu at (162.8, 109.9)
- added REF**: PROTO_HOLE, One_Month_Footprints:PROTO_HOLE, F.Cu at (160.3, 109.9)
- added REF**: PROTO_HOLE, One_Month_Footprints:PROTO_HOLE, F.Cu at (157.7, 109.9)
- added REF**: PROTO_HOLE, One_Month_Footprints:PROTO_HOLE, F.Cu at (99.3, 114.9)
- added REF**: PROTO_HOLE, One_Month_Footprints:PROTO_HOLE, F.Cu at (155.2, 109.9)
- added REF**: PROTO_HOLE, One_Month_Footprints:PROTO_HOLE, F.Cu at (152.7, 109.9)
- added REF**: PROTO_HOLE, One_Month_Footprints:PROTO_HOLE, F.Cu at (150.1, 109.9)
- added REF**: PROTO_HOLE, One_Month_Footprints:PROTO_HOLE, F.Cu at (147.6, 109.9)
- added REF**: PROTO_HOLE, One_Month_Footprints:PROTO_HOLE, F.Cu at (145.0, 109.9)
- added REF**: PROTO_HOLE, One_Month_Footprints:PROTO_HOLE, F.Cu at (142.5, 109.9)
- added REF**: PROTO_HOLE, One_Month_Footprints:PROTO_HOLE, F.Cu at (140.0, 109.9)
- added REF**: PROTO_HOLE, One_Month_Footprints:PROTO_HOLE, F.Cu at (137.4, 109.9)
- added REF**: PROTO_HOLE, One_Month_Footprints:PROTO_HOLE, F.Cu at (134.9, 109.9)
- added REF**: PROTO_HOLE, One_Month_Footprints:PROTO_HOLE, F.Cu at (132.3, 109.9)
- added REF**: PROTO_HOLE, One_Month_Footprints:PROTO_HOLE, F.Cu at (119.6, 112.4)
- added REF**: PROTO_HOLE, One_Month_Footprints:PROTO_HOLE, F.Cu at (129.8, 109.9)
- added REF**: PROTO_HOLE, One_Month_Footprints:PROTO_HOLE, F.Cu at (127.3, 109.9)
- added REF**: PROTO_HOLE, One_Month_Footprints:PROTO_HOLE, F.Cu at (124.7, 109.9)
- added REF**: PROTO_HOLE, One_Month_Footprints:PROTO_HOLE, F.Cu at (122.2, 109.9)
- added REF**: PROTO_HOLE, One_Month_Footprints:PROTO_HOLE, F.Cu at (195.8, 107.3)
- added REF**: PROTO_HOLE, One_Month_Footprints:PROTO_HOLE, F.Cu at (193.3, 107.3)
- added REF**: PROTO_HOLE, One_Month_Footprints:PROTO_HOLE, F.Cu at (190.8, 107.3)
- added REF**: PROTO_HOLE, One_Month_Footprints:PROTO_HOLE, F.Cu at (188.2, 107.3)
- added REF**: PROTO_HOLE, One_Month_Footprints:PROTO_HOLE, F.Cu at (185.7, 107.3)
- added REF**: PROTO_HOLE, One_Month_Footprints:PROTO_HOLE, F.Cu at (183.1, 107.3)
- added REF**: PROTO_HOLE, One_Month_Footprints:PROTO_HOLE, F.Cu at (117.1, 112.4)
- added REF**: PROTO_HOLE, One_Month_Footprints:PROTO_HOLE, F.Cu at (180.6, 107.3)
- added REF**: PROTO_HOLE, One_Month_Footprints:PROTO_HOLE, F.Cu at (178.1, 107.3)
- added REF**: PROTO_HOLE, One_Month_Footprints:PROTO_HOLE, F.Cu at (175.5, 107.3)
- added REF**: PROTO_HOLE, One_Month_Footprints:PROTO_HOLE, F.Cu at (173.0, 107.3)
- added REF**: PROTO_HOLE, One_Month_Footprints:PROTO_HOLE, F.Cu at (170.4, 107.3)
- added REF**: PROTO_HOLE, One_Month_Footprints:PROTO_HOLE, F.Cu at (167.9, 107.3)
- added REF**: PROTO_HOLE, One_Month_Footprints:PROTO_HOLE, F.Cu at (165.4, 107.3)
- added REF**: PROTO_HOLE, One_Month_Footprints:PROTO_HOLE, F.Cu at (162.8, 107.3)
- added REF**: PROTO_HOLE, One_Month_Footprints:PROTO_HOLE, F.Cu at (160.3, 107.3)
- added REF**: PROTO_HOLE, One_Month_Footprints:PROTO_HOLE, F.Cu at (157.7, 107.3)
- added REF**: PROTO_HOLE, One_Month_Footprints:PROTO_HOLE, F.Cu at (114.6, 112.4)
- added REF**: PROTO_HOLE, One_Month_Footprints:PROTO_HOLE, F.Cu at (155.2, 107.3)
- added REF**: PROTO_HOLE, One_Month_Footprints:PROTO_HOLE, F.Cu at (152.7, 107.3)
- added REF**: PROTO_HOLE, One_Month_Footprints:PROTO_HOLE, F.Cu at (150.1, 107.3)
- added REF**: PROTO_HOLE, One_Month_Footprints:PROTO_HOLE, F.Cu at (147.6, 107.3)
- added REF**: PROTO_HOLE, One_Month_Footprints:PROTO_HOLE, F.Cu at (145.0, 107.3)
- added REF**: PROTO_HOLE, One_Month_Footprints:PROTO_HOLE, F.Cu at (142.5, 107.3)
- added REF**: PROTO_HOLE, One_Month_Footprints:PROTO_HOLE, F.Cu at (140.0, 107.3)
- added REF**: PROTO_HOLE, One_Month_Footprints:PROTO_HOLE, F.Cu at (137.4, 107.3)
- added REF**: PROTO_HOLE, One_Month_Footprints:PROTO_HOLE, F.Cu at (134.9, 107.3)
- added REF**: PROTO_HOLE, One_Month_Footprints:PROTO_HOLE, F.Cu at (132.3, 107.3)
- added REF**: PROTO_HOLE, One_Month_Footprints:PROTO_HOLE, F.Cu at (112.0, 112.4)
- added REF**: PROTO_HOLE, One_Month_Footprints:PROTO_HOLE, F.Cu at (129.8, 107.3)
- added REF**: PROTO_HOLE, One_Month_Footprints:PROTO_HOLE, F.Cu at (127.3, 107.3)
- added REF**: PROTO_HOLE, One_Month_Footprints:PROTO_HOLE, F.Cu at (124.7, 107.3)
- added REF**: PROTO_HOLE, One_Month_Footprints:PROTO_HOLE, F.Cu at (122.2, 107.3)
- added REF**: PROTO_HOLE, One_Month_Footprints:PROTO_HOLE, F.Cu at (188.2, 104.8)
- added REF**: PROTO_HOLE, One_Month_Footprints:PROTO_HOLE, F.Cu at (185.7, 104.8)
- added REF**: PROTO_HOLE, One_Month_Footprints:PROTO_HOLE, F.Cu at (183.1, 104.8)
- added REF**: PROTO_HOLE, One_Month_Footprints:PROTO_HOLE, F.Cu at (180.6, 104.8)
- added REF**: PROTO_HOLE, One_Month_Footprints:PROTO_HOLE, F.Cu at (178.1, 104.8)
- added REF**: PROTO_HOLE, One_Month_Footprints:PROTO_HOLE, F.Cu at (175.5, 104.8)
- added REF**: PROTO_HOLE, One_Month_Footprints:PROTO_HOLE, F.Cu at (109.5, 112.4)
- added REF**: PROTO_HOLE, One_Month_Footprints:PROTO_HOLE, F.Cu at (173.0, 104.8)
- added REF**: PROTO_HOLE, One_Month_Footprints:PROTO_HOLE, F.Cu at (170.4, 104.8)
- added REF**: PROTO_HOLE, One_Month_Footprints:PROTO_HOLE, F.Cu at (167.9, 104.8)
- added REF**: PROTO_HOLE, One_Month_Footprints:PROTO_HOLE, F.Cu at (165.4, 104.8)
- added REF**: PROTO_HOLE, One_Month_Footprints:PROTO_HOLE, F.Cu at (162.8, 104.8)
- added REF**: PROTO_HOLE, One_Month_Footprints:PROTO_HOLE, F.Cu at (160.3, 104.8)
- added REF**: PROTO_HOLE, One_Month_Footprints:PROTO_HOLE, F.Cu at (157.7, 104.8)
- added REF**: PROTO_HOLE, One_Month_Footprints:PROTO_HOLE, F.Cu at (155.2, 104.8)
- added REF**: PROTO_HOLE, One_Month_Footprints:PROTO_HOLE, F.Cu at (152.7, 104.8)
- added REF**: PROTO_HOLE, One_Month_Footprints:PROTO_HOLE, F.Cu at (150.1, 104.8)
- added REF**: PROTO_HOLE, One_Month_Footprints:PROTO_HOLE, F.Cu at (106.9, 112.4)
- added REF**: PROTO_HOLE, One_Month_Footprints:PROTO_HOLE, F.Cu at (147.6, 104.8)
- added REF**: PROTO_HOLE, One_Month_Footprints:PROTO_HOLE, F.Cu at (145.0, 104.8)
- added REF**: PROTO_HOLE, One_Month_Footprints:PROTO_HOLE, F.Cu at (142.5, 104.8)
- added REF**: PROTO_HOLE, One_Month_Footprints:PROTO_HOLE, F.Cu at (140.0, 104.8)
- added REF**: PROTO_HOLE, One_Month_Footprints:PROTO_HOLE, F.Cu at (137.4, 104.8)
- added REF**: PROTO_HOLE, One_Month_Footprints:PROTO_HOLE, F.Cu at (134.9, 104.8)
- added REF**: PROTO_HOLE, One_Month_Footprints:PROTO_HOLE, F.Cu at (132.3, 104.8)
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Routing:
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- added copper zone on F.Cu, net +3V3
- added copper zone on B.Cu, net GND
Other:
- board size 59.1 x 53.3 mm -> 102.5 x 66 mm
- board text removed: "+"
- board text removed: "-"
